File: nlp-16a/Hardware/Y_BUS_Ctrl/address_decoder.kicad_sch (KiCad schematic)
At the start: 20 parts, among them U41 CD74HC00, U42 CD74HC00

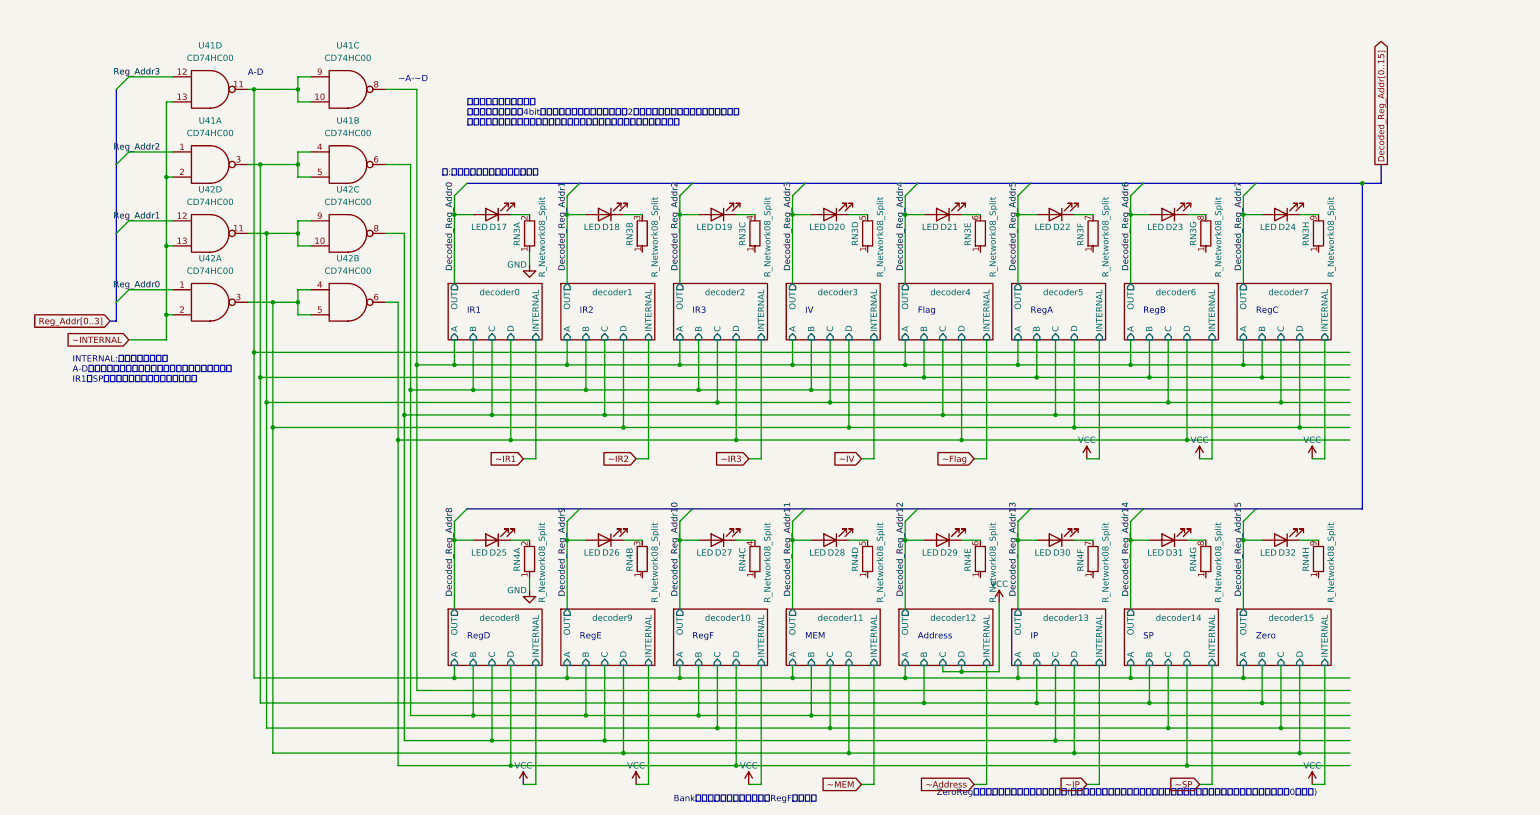
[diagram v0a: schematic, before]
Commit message: Y BUS制御 更新
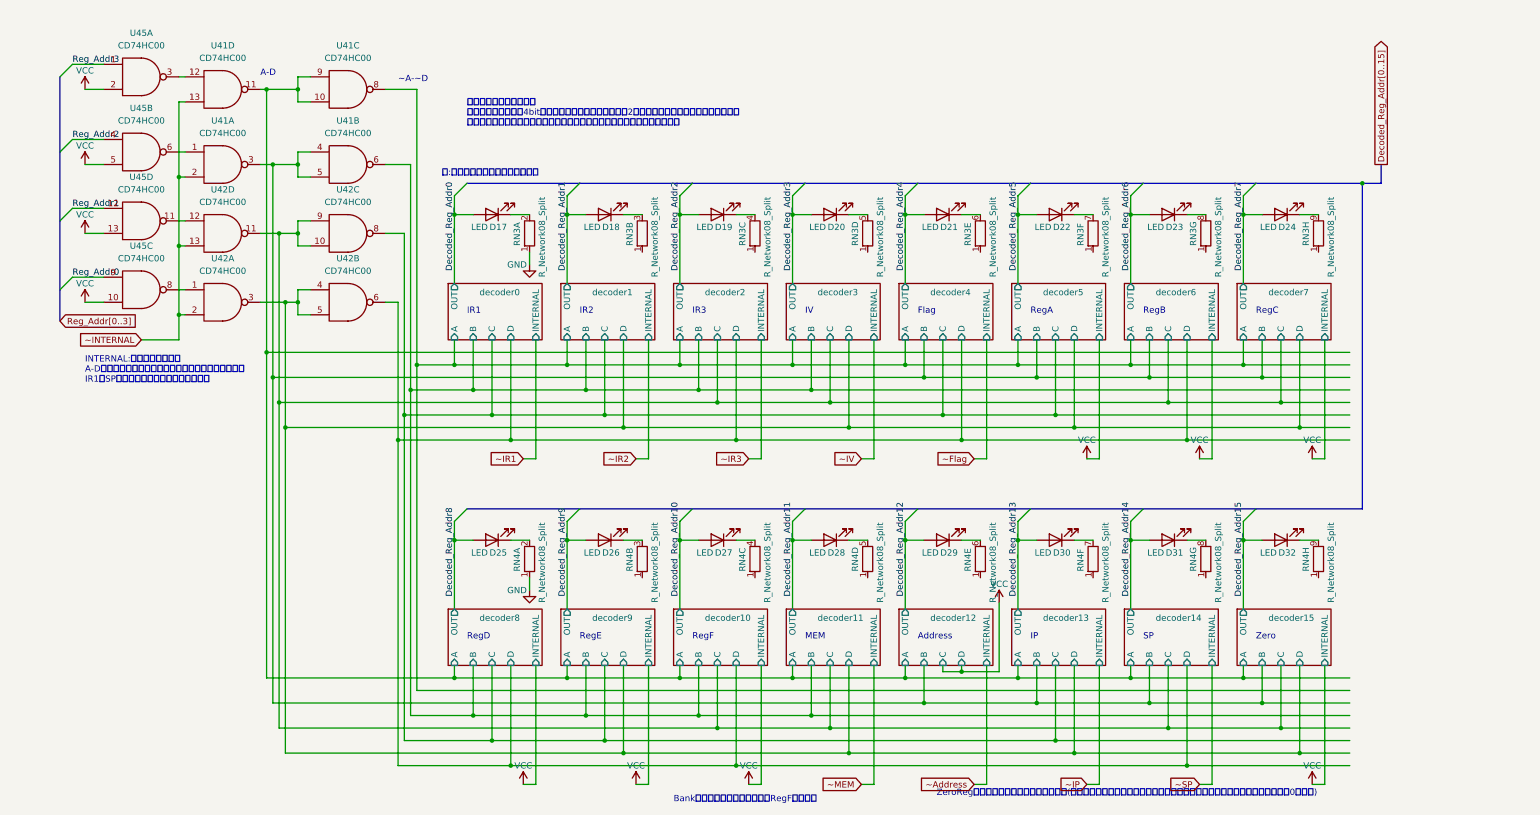
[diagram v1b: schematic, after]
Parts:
- added U45: CD74HC00, Package_DIP:DIP-14_W7.62mm, symbol CD74HCXX:CD74HC00
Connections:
- net GND: now also U45.7 (GND), U45.7 (GND), U45.7 (GND), U45.7 (GND)
- net Reg_Addr0: now also U45.9; no longer U42.1
- net Reg_Addr1: now also U45.12; no longer U42.12
- net Reg_Addr2: now also U45.4; no longer U41.1
- net Reg_Addr3: now also U45.1; no longer U41.12
- net VCC: now also U45.10, U45.13, U45.14 (VCC), U45.14 (VCC), U45.14 (VCC), U45.14 (VCC), U45.2, U45.5
- new net: U41.1, U45.6
- new net: U42.12, U45.11
- new net: U42.1, U45.8
- new net: U41.12, U45.3
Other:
- moved on the sheet: U41A, U41D, U42A, U42D
